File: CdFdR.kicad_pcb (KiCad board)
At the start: 2 copper layers, 64.8 x 90.2 mm, 17 parts, among them J1 Moteur_1, J2 Moteur_2, J3 Moteur_3, J4 Moteur_4, U1 ESP32-S3-N16R8-DEVBOARD

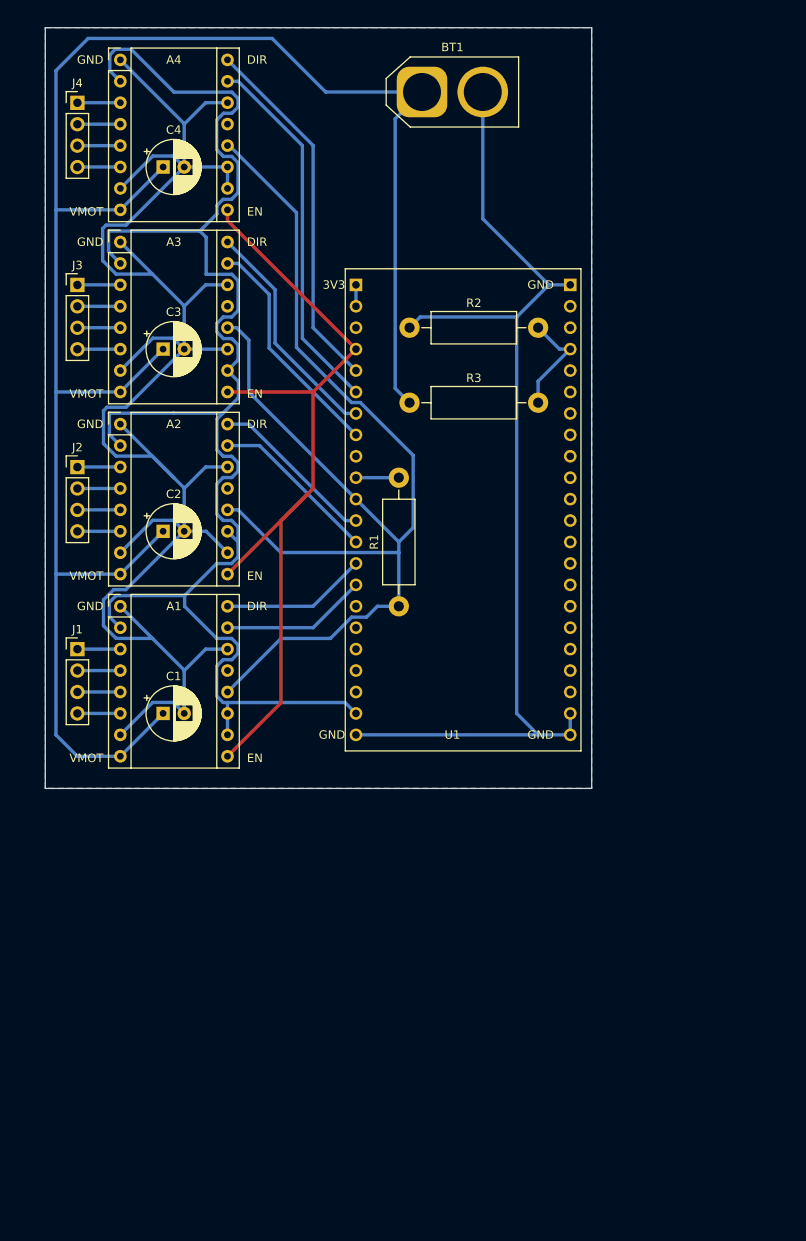
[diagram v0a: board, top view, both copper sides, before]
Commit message: Version envoyé pour vérif
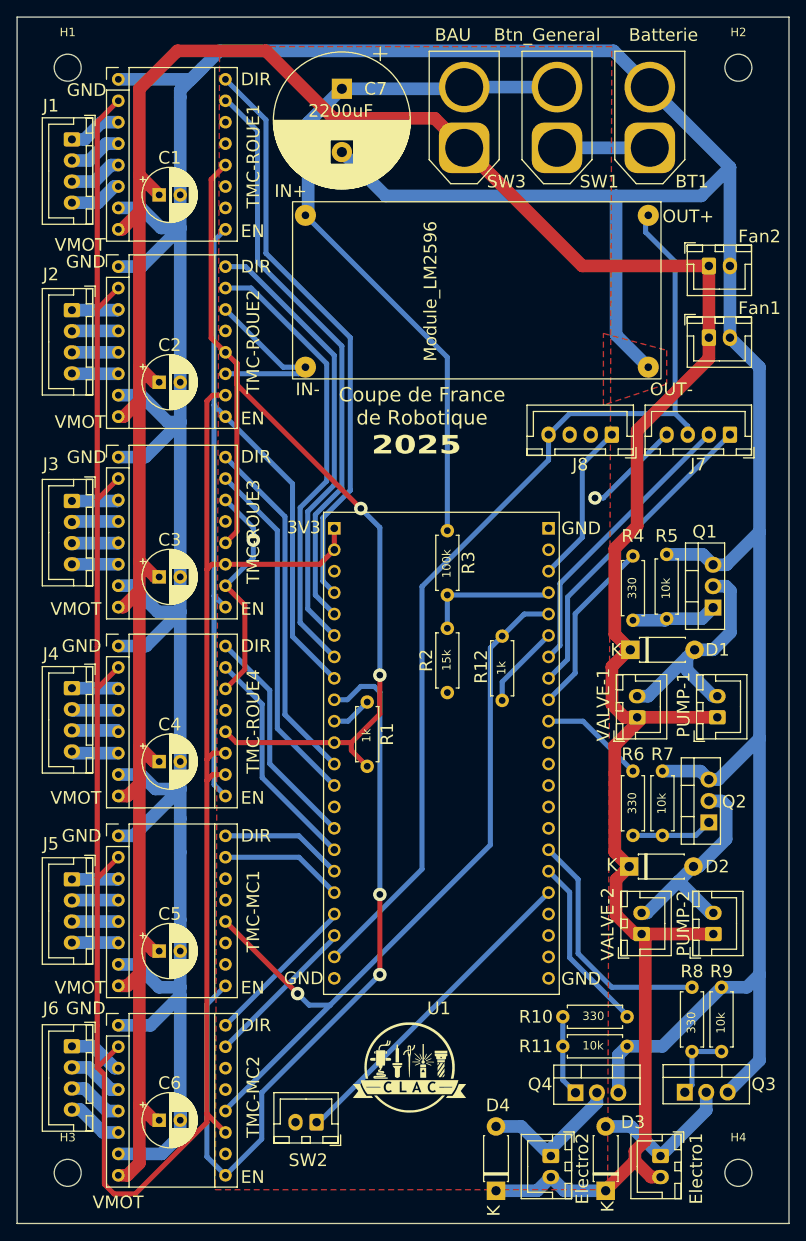
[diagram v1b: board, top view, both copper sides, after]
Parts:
- added C5: 100uF/35V, Capacitor_THT:CP_Radial_D6.3mm_P2.50mm, F.Cu at (66.8, 157.7)
- added C6: 100uF/35V, Capacitor_THT:CP_Radial_D6.3mm_P2.50mm, F.Cu at (66.8, 177.8)
- added C7: 2200 uF, Capacitor_THT:CP_Radial_D16.0mm_P7.50mm, F.Cu at (88.5, 55.5)
- added D1: FR107, Diode_THT:D_DO-41_SOD81_P7.62mm_Horizontal, F.Cu at (122.7, 122.0)
- added D2: FR107, Diode_THT:D_DO-41_SOD81_P7.62mm_Horizontal, F.Cu at (122.6, 147.7)
- added D3: FR107, Diode_THT:D_DO-41_SOD81_P7.62mm_Horizontal, F.Cu at (119.8, 186.1)
- added D4: FR107, Diode_THT:D_DO-41_SOD81_P7.62mm_Horizontal, F.Cu at (106.8, 186.1)
- added Electro1: ElectroAimant, Connector_JST:JST_XH_B2B-XH-A_1x02_P2.50mm_Vertical, F.Cu at (126.3, 182.0)
- added Electro2: ElectroAimant, Connector_JST:JST_XH_B2B-XH-A_1x02_P2.50mm_Vertical, F.Cu at (113.3, 182.0)
- added Fan1: Fan, Connector_JST:JST_XH_B2B-XH-A_1x02_P2.50mm_Vertical, F.Cu at (132.0, 85.0)
- added Fan2: Fan, Connector_JST:JST_XH_B2B-XH-A_1x02_P2.50mm_Vertical, F.Cu at (132.0, 76.5)
- added G***: LOGO, LOGO, F.Cu at (96.5, 171.5)
- added H1: MountingHole, MountingHole:MountingHole_3.2mm_M3, F.Cu at (56.0, 53.0)
- added H2: MountingHole, MountingHole:MountingHole_3.2mm_M3, F.Cu at (135.5, 53.0)
- added H3: MountingHole, MountingHole:MountingHole_3.2mm_M3, F.Cu at (56.0, 184.0)
- added H4: MountingHole, MountingHole:MountingHole_3.2mm_M3, F.Cu at (135.5, 184.0)
- added J5: Nema17_5, Connector_JST:JST_XH_B4B-XH-A_1x04_P2.50mm_Vertical, F.Cu at (56.5, 149.2)
- added J6: Nema17_6, Connector_JST:JST_XH_B4B-XH-A_1x04_P2.50mm_Vertical, F.Cu at (56.5, 169.0)
- added J7: IHM, Connector_JST:JST_XH_B4B-XH-A_1x04_P2.50mm_Vertical, F.Cu at (134.5, 96.5)
- added J8: Lidar, Connector_JST:JST_XH_B4B-XH-A_1x04_P2.50mm_Vertical, F.Cu at (120.5, 96.5)
- added Module_LM2596: LM2596, Custom:LM2596 Converter DC-DC, F.Cu at (104.5, 79.5)
- added PUMP-1: PUMP, Connector_JST:JST_XH_B2B-XH-A_1x02_P2.50mm_Vertical, F.Cu at (133.0, 130.0)
- added PUMP-2: PUMP, Connector_JST:JST_XH_B2B-XH-A_1x02_P2.50mm_Vertical, F.Cu at (132.5, 155.7)
- added Q1: IRLZ44N, Package_TO_SOT_THT:TO-220-3_Vertical, F.Cu at (132.5, 117.0)
- added Q2: IRLZ44N, Package_TO_SOT_THT:TO-220-3_Vertical, F.Cu at (132.0, 142.5)
- added Q3: IRLZ44N, Package_TO_SOT_THT:TO-220-3_Vertical, F.Cu at (129.2, 174.4)
- added Q4: IRLZ44N, Package_TO_SOT_THT:TO-220-3_Vertical, F.Cu at (116.2, 174.5)
- added R10: 330, Resistor_THT:R_Axial_DIN0207_L6.3mm_D2.5mm_P7.62mm_Horizontal, F.Cu at (122.3, 165.5)
- added R11: 10k, Resistor_THT:R_Axial_DIN0207_L6.3mm_D2.5mm_P7.62mm_Horizontal, F.Cu at (122.3, 169.0)
- added R12: 1k, Resistor_THT:R_Axial_DIN0207_L6.3mm_D2.5mm_P7.62mm_Horizontal, F.Cu at (107.5, 120.4)
- added R4: 330, Resistor_THT:R_Axial_DIN0207_L6.3mm_D2.5mm_P7.62mm_Horizontal, F.Cu at (123.0, 110.9)
- added R5: 10k, Resistor_THT:R_Axial_DIN0207_L6.3mm_D2.5mm_P7.62mm_Horizontal, F.Cu at (127.0, 110.7)
- added R6: 330, Resistor_THT:R_Axial_DIN0207_L6.3mm_D2.5mm_P7.62mm_Horizontal, F.Cu at (123.0, 136.4)
- added R7: 10k, Resistor_THT:R_Axial_DIN0207_L6.3mm_D2.5mm_P7.62mm_Horizontal, F.Cu at (126.5, 136.4)
- added R8: 330, Resistor_THT:R_Axial_DIN0207_L6.3mm_D2.5mm_P7.62mm_Horizontal, F.Cu at (130.0, 162.0)
- added R9: 10k, Resistor_THT:R_Axial_DIN0207_L6.3mm_D2.5mm_P7.62mm_Horizontal, F.Cu at (133.5, 162.0)
- added SW1: Alim_generale, Connector_AMASS:AMASS_XT60-F_1x02_P7.20mm_Vertical, F.Cu at (114.0, 62.5)
- added SW2: Tirette, Connector_JST:JST_XH_B2B-XH-A_1x02_P2.50mm_Vertical, F.Cu at (85.5, 178.0)
- added SW3: Urgence, Connector_AMASS:AMASS_XT60-F_1x02_P7.20mm_Vertical, F.Cu at (103.0, 62.5)
- added TMC-MC1: Pololu_Breakout, Custom:Pololu_Breakout-16_15.2x20.3mm_Better_Silkscreen, F.Cu at (62.0, 144.1)
- added TMC-MC2: Pololu_Breakout, Custom:Pololu_Breakout-16_15.2x20.3mm_Better_Silkscreen, F.Cu at (62.0, 166.5)
- added VALVE-1: VALVE, Connector_JST:JST_XH_B2B-XH-A_1x02_P2.50mm_Vertical, F.Cu at (123.5, 130.0)
- added VALVE-2: VALVE, Connector_JST:JST_XH_B2B-XH-A_1x02_P2.50mm_Vertical, F.Cu at (124.0, 155.7)
- J1: value Moteur_1 -> Nema17_1; footprint Connector_PinHeader_2.54mm:PinHeader_1x04_P2.54mm_Vertical -> Connector_JST:JST_XH_B4B-XH-A_1x04_P2.50mm_Vertical
- J2: value Moteur_2 -> Nema17_2; footprint Connector_PinHeader_2.54mm:PinHeader_1x04_P2.54mm_Vertical -> Connector_JST:JST_XH_B4B-XH-A_1x04_P2.50mm_Vertical
- J3: value Moteur_3 -> Nema17_3; footprint Connector_PinHeader_2.54mm:PinHeader_1x04_P2.54mm_Vertical -> Connector_JST:JST_XH_B4B-XH-A_1x04_P2.50mm_Vertical
- J4: value Moteur_4 -> Nema17_4; footprint Connector_PinHeader_2.54mm:PinHeader_1x04_P2.54mm_Vertical -> Connector_JST:JST_XH_B4B-XH-A_1x04_P2.50mm_Vertical
- R1, R2, R3: footprint Resistor_THT:R_Axial_DIN0411_L9.9mm_D3.6mm_P15.24mm_Horizontal -> Resistor_THT:R_Axial_DIN0207_L6.3mm_D2.5mm_P7.62mm_Horizontal
- TMC-ROUE1: renamed from A1; value M4 -> Pololu_Breakout
- TMC-ROUE2: renamed from A2; value M3 -> Pololu_Breakout
- TMC-ROUE3: renamed from A3; value M2 -> Pololu_Breakout
- TMC-ROUE4: renamed from A4; value M1 -> Pololu_Breakout
- moved C4 70.5 mm to (66.8, 135.2)
- moved TMC-ROUE4 69.5 mm to (62.0, 121.5)
- moved J4 69.4 mm to (56.5, 126.5), turned to -90 degrees
- moved TMC-ROUE1 62.5 mm to (62.0, 54.4)
- moved C1 61.5 mm to (66.8, 68.1)
- moved J1 60.4 mm to (56.5, 61.5), turned to -90 degrees
- moved R2 43.5 mm to (101.0, 127.1), turned to 90 degrees
- moved U1 29.0 mm to (87.6, 107.6)
- moved BT1 27.8 mm to (125.0, 62.5), turned to 90 degrees
- moved C3 27.0 mm to (66.8, 113.4)
- moved J3 25.6 mm to (56.5, 104.4), turned to -90 degrees
- moved TMC-ROUE3 25.5 mm to (62.0, 99.2)
- moved TMC-ROUE2 18.7 mm to (62.0, 76.6)
- moved J2 18.6 mm to (56.5, 81.7), turned to -90 degrees
- moved C2 17.7 mm to (66.8, 90.3)
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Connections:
- BT1 pad 1: +BATT -> Net-(BT1-+)
- C1 pad 1: +BATT -> +24V
- C2 pad 1: +BATT -> +24V
- C3 pad 1: +BATT -> +24V
- C4 pad 1: +BATT -> +24V
- R1 pad 1: UART_Mot -> Net-(U1-17)
- R1 pad 2: /TX1 -> UART_Mot
- R3 pad 1: +BATT -> V_Batt
- TMC-ROUE1 pad 10: +5V -> GND
- TMC-ROUE1 pad 11: +5V -> GND
- TMC-ROUE1 pad 15: M4_STP -> M1_STP
- TMC-ROUE1 pad 16: M4_DIR -> M1_DIR
- TMC-ROUE1 pad 2: +5V -> +3.3V
- TMC-ROUE1 pad 8: +BATT -> +24V
- TMC-ROUE2 pad 10: GND -> +3.3V
- TMC-ROUE2 pad 11: +5V -> GND
- TMC-ROUE2 pad 15: M3_STP -> M2_STP
- TMC-ROUE2 pad 16: M3_DIR -> M2_DIR
- TMC-ROUE2 pad 2: +5V -> +3.3V
- TMC-ROUE2 pad 8: +BATT -> +24V
- TMC-ROUE3 pad 10: +5V -> GND
- TMC-ROUE3 pad 11: GND -> +3.3V
- TMC-ROUE3 pad 15: M2_STP -> M3_STP
- TMC-ROUE3 pad 16: M2_DIR -> M3_DIR
- TMC-ROUE3 pad 2: +5V -> +3.3V
- TMC-ROUE3 pad 8: +BATT -> +24V
- TMC-ROUE4 pad 10: GND -> +3.3V
- TMC-ROUE4 pad 11: GND -> +3.3V
- TMC-ROUE4 pad 15: M1_STP -> M4_STP
- TMC-ROUE4 pad 16: M1_DIR -> M4_DIR
- TMC-ROUE4 pad 2: +5V -> +3.3V
- TMC-ROUE4 pad 8: +BATT -> +24V
- U1 pad 1: Net-(U1-3V3-Pad1) -> +3.3V
- U1 pad 10: /TX1 -> Net-(U1-17)
- U1 pad 14: M4_DIR -> unconnected-(U1-46-Pad14)
- U1 pad 15: M4_STP -> M4_DIR
- U1 pad 16: unconnected-(U1-10-Pad16) -> M4_STP
- U1 pad 17: unconnected-(U1-11-Pad17) -> M5_DIR
- U1 pad 18: unconnected-(U1-12-Pad18) -> M5_STP
- U1 pad 19: unconnected-(U1-13-Pad19) -> M6_DIR
- U1 pad 2: Net-(U1-3V3-Pad1) -> +3.3V
- U1 pad 20: unconnected-(U1-14-Pad20) -> M6_STP
- U1 pad 27: unconnected-(U1-21-Pad27) -> Net-(U1-21)
- U1 pad 28: unconnected-(U1-47-Pad28) -> ELECTRO2
- U1 pad 29: unconnected-(U1-48-Pad29) -> ELECTRO1
- U1 pad 35: unconnected-(U1-38-Pad35) -> PUMP_VALVE2
- U1 pad 36: unconnected-(U1-39-Pad36) -> PUMP_VALVE1
- U1 pad 37: unconnected-(U1-40-Pad37) -> CLK_IHM
- U1 pad 38: unconnected-(U1-41-Pad38) -> DIO_IHM
- U1 pad 39: unconnected-(U1-42-Pad39) -> Net-(U1-42)
- U1 pad 4: Drive_Mot_EN -> M1_DIR
- U1 pad 40: unconnected-(U1-2-Pad40) -> UART_Chariot
- U1 pad 42: unconnected-(U1-44-Pad42) -> TX_Lidar
- U1 pad 5: M1_DIR -> M1_STP
- U1 pad 6: M1_STP -> M2_DIR
- U1 pad 7: M2_DIR -> M2_STP
- U1 pad 8: M2_STP -> Drive_Mot_EN
- U1 pad 9: unconnected-(U1-16-Pad9) -> Drive_Chariot_EN
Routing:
- net +24V: track 0.00 -> 412.2 mm
- net +3.3V: track 0.00 -> 278.3 mm
- net GND: track 343.6 -> 601.6 mm, vias 0 -> 2
- net +BATT: track 225.5 -> 0.00 mm
- net Drive_Chariot_EN: track 0.00 -> 95.5 mm, vias 0 -> 2
- net UART_Chariot: track 0.00 -> 93.0 mm, vias 0 -> 1
- net V_Batt: track 0.00 -> 87.2 mm
- net +5V: track 190.0 -> 117.5 mm
- net Net-(U1-21): track 0.00 -> 38.5 mm
- net CLK_IHM: track 0.00 -> 37.8 mm
- net DIO_IHM: track 0.00 -> 34.2 mm
- net ELECTRO1: track 0.00 -> 28.9 mm
- net Net-(D1-A): track 0.00 -> 27.8 mm
- net UART_Mot: track 146.5 -> 119.8 mm, vias 0 -> 2
- net M2_STP: track 27.4 -> 53.5 mm
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- added copper zone on F.Cu, net GND
- removed copper zone on B.Cu, net GND
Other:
- board size 64.8 x 90.2 mm -> 91.5 x 143 mm
- board text added: "100k"
- board text added: "10k"
- board text added: "15k"
- board text added: "1k"
- board text added: "2025"
- board text added: "2200uF"
- board text added: "330"
- board text added: "BAU"
- board text added: "Batterie"
- board text added: "Btn_General"
- board text added: "Coupe de France de Robotique"
- board text added: "DIR"
